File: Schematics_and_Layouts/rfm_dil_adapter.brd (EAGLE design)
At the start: 31.8 x 22.9 mm, 17 parts

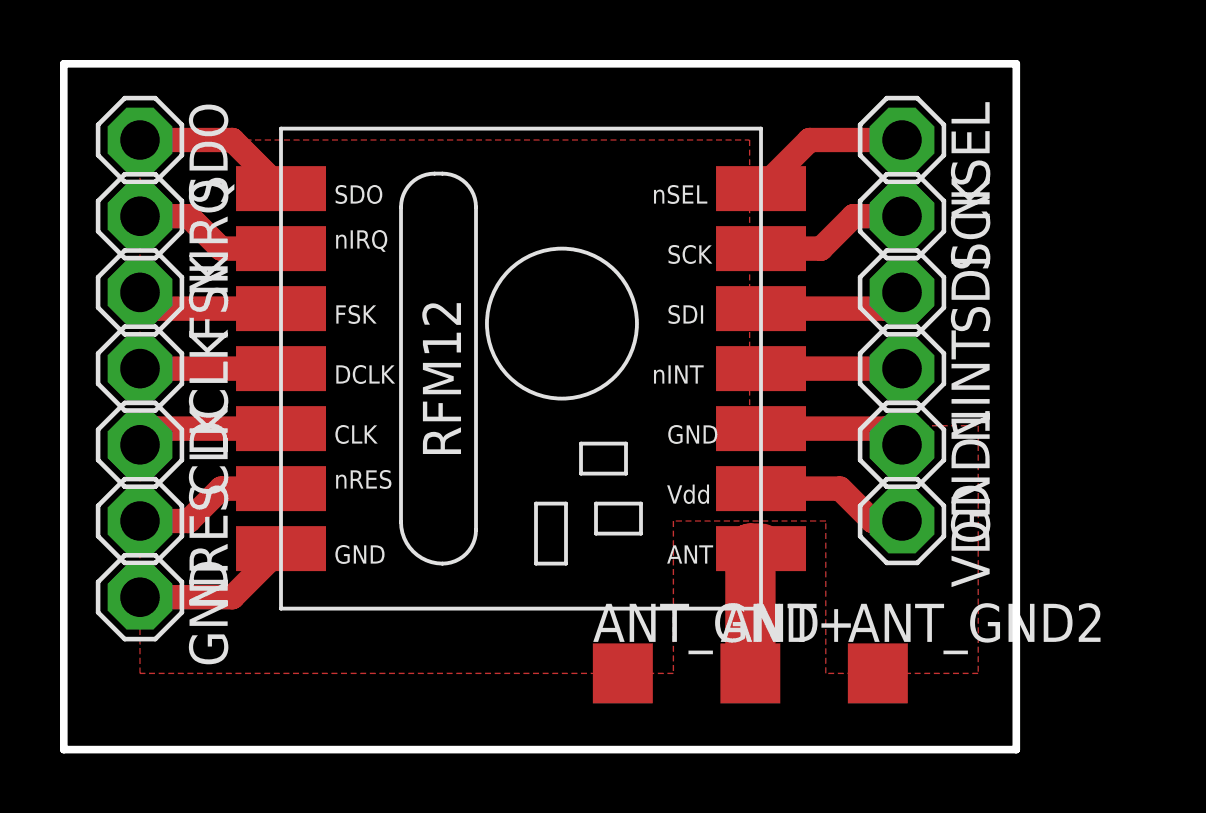
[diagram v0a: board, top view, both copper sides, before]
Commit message: Added Gerber Files
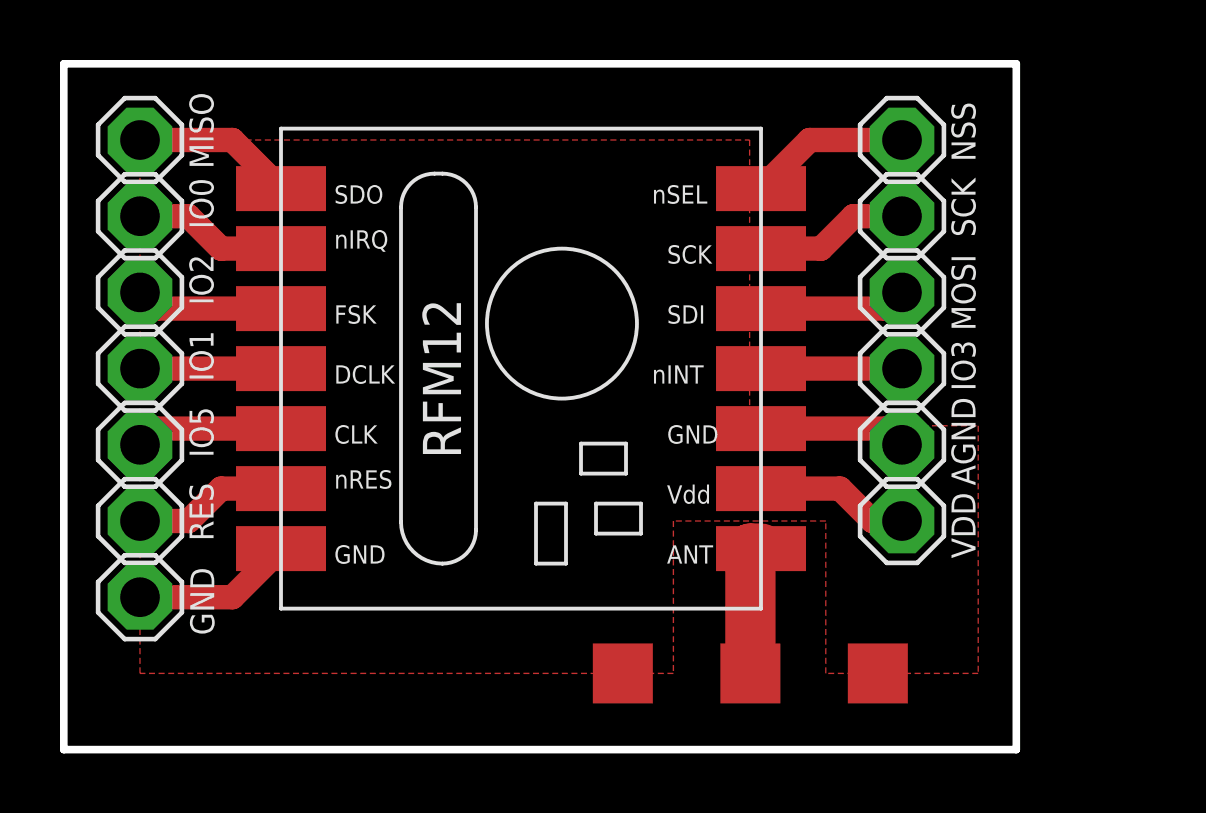
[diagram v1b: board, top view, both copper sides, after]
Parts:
- renumbered CLK to IO5, DCLK to IO1, FSK to IO2, GND1 to AGND, NINT to IO3, NIRQ to IO0, NRES to RES, NSEL to NSS, SDI to MOSI, SDO to MISO
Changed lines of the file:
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@@
 <?xml version="1.0" encoding="utf-8"?>
 <!DOCTYPE eagle SYSTEM "eagle.dtd">
-<eagle version="6.3">
+<eagle version="6.6.0">
 <drawing>
 <settings>
@@
 <setting verticaltext="up"/>
 </settings>
-<grid distance="1.27" unitdist="mm" unit="mm" style="lines" multiple="1" display="yes" altdistance="25" altunitdist="mil" altunit="mil"/>
+<grid distance="1.27" unitdist="mm" unit="mm" style="lines" multiple="1" display="yes" altdistance="12.5" altunitdist="mil" altunit="mil"/>
 <layers>
 <layer number="1" name="Top" color="4" fill="1" visible="yes" active="yes"/>
@@
 </autorouter>
 <elements>
-<element name="U$1" library="fp" package="RFM12_Z" value="RFM12_Z" x="15.24" y="12.7" rot="R270"/>
-<element name="CLK" library="solpad" package="SE13" value="SE13" x="2.54" y="10.16" rot="R270"/>
-<element name="DCLK" library="solpad" package="SE13" value="SE13" x="2.54" y="12.7" rot="R270"/>
-<element name="FSK" library="solpad" package="SE13" value="SE13" x="2.54" y="15.24" rot="R270"/>
-<element name="SDI" library="solpad" package="SE13" value="SE13" x="27.94" y="15.24" rot="R270"/>
-<element name="SDO" library="solpad" package="SE13" value="SE13" x="2.54" y="20.32" rot="R270"/>
-<element name="SCK" library="solpad" package="SE13" value="SE13" x="27.94" y="17.78" rot="R270"/>
-<element name="NSEL" library="solpad" package="SE13" value="SE13" x="27.94" y="20.32" rot="R270"/>
-<element name="GND" library="solpad" package="SE13" value="SE13" x="2.54" y="5.08" rot="R270"/>
-<element name="GND1" library="solpad" package="SE13" value="SE13" x="27.94" y="10.16" rot="R270"/>
-<element name="NRES" library="solpad" package="SE13" value="SE13" x="2.54" y="7.62" rot="R270"/>
-<element name="NIRQ" library="solpad" package="SE13" value="SE13" x="2.54" y="17.78" rot="R270"/>
-<element name="NINT" library="solpad" package="SE13" value="SE13" x="27.94" y="12.7" rot="R270"/>
-<element name="VDD" library="solpad" package="SE13" value="SE13" x="27.94" y="7.62" rot="R270"/>
-<element name="ANT+" library="testpad" package="TP20SQ" value="PTR1TP20SQ" x="22.885" y="2.54">
-<attribute name="TP_SIGNAL_NAME" value="" x="22.885" y="2.54" size="1.778" layer="27" display="off"/>
-</element>
-<element name="ANT_GND" library="testpad" package="TP20SQ" value="PTR1TP20SQ" x="18.635" y="2.54">
-<attribute name="TP_SIGNAL_NAME" value="" x="18.635" y="2.54" size="1.778" layer="27" display="off"/>
-</element>
-<element name="ANT_GND2" library="testpad" package="TP20SQ" value="PTR1TP20SQ" x="27.135" y="2.54">
-<attribute name="TP_SIGNAL_NAME" value="" x="27.135" y="2.54" size="1.778" layer="27" display="off"/>
+<element name="U$1" library="fp" package="RFM12_Z" value="RFM12_Z" x="15.24" y="12.7" smashed="yes" rot="R270"/>
+<element name="IO5" library="solpad" package="SE13" value="SE13" x="2.54" y="10.16" smashed="yes" rot="R270">
+<attribute name="NAME" x="4.191" y="11.43" size="0.8" layer="25" font="vector" ratio="20" rot="R270"/>
+</element>
+<element name="IO1" library="solpad" package="SE13" value="SE13" x="2.54" y="12.7" smashed="yes" rot="R270">
+<attribute name="NAME" x="4.191" y="13.97" size="0.8" layer="25" font="vector" ratio="20" rot="R270"/>
+</element>
+<element name="IO2" library="solpad" package="SE13" value="SE13" x="2.54" y="15.24" smashed="yes" rot="R270">
+<attribute name="NAME" x="4.191" y="16.51" size="0.8" layer="25" font="vector" ratio="20" rot="R270"/>
+</element>
+<element name="MOSI" library="solpad" package="SE13" value="SE13" x="27.94" y="15.24" smashed="yes" rot="R270">
+<attribute name="NAME" x="29.591" y="16.51" size="0.8" layer="25" font="vector" ratio="20" rot="R270"/>
+</element>
+<element name="MISO" library="solpad" package="SE13" value="SE13" x="2.54" y="20.32" smashed="yes" rot="R270">
+<attribute name="NAME" x="4.191" y="21.9075" size="0.8" layer="25" font="vector" ratio="20" rot="R270"/>
+</element>
+<element name="SCK" library="solpad" package="SE13" value="SE13" x="27.94" y="17.78" smashed="yes" rot="R270">
+<attribute name="NAME" x="29.591" y="19.05" size="0.8" layer="25" font="vector" ratio="20" rot="R270"/>
+</element>
+<element name="NSS" library="solpad" package="SE13" value="SE13" x="27.94" y="20.32" smashed="yes" rot="R270">
+<attribute name="NAME" x="29.591" y="21.59" size="0.8" layer="25" font="vector" ratio="20" rot="R270"/>
+</element>
+<element name="GND" library="solpad" package="SE13" value="SE13" x="2.54" y="5.08" smashed="yes" rot="R270">
+<attribute name="NAME" x="5.0165" y="3.81" size="0.8" layer="25" font="vector" ratio="20" rot="R90"/>
+</element>
+<element name="AGND" library="solpad" package="SE13" value="SE13" x="27.94" y="10.16" smashed="yes" rot="R270">
+<attribute name="NAME" x="29.591" y="11.7475" size="0.8" layer="25" font="vector" ratio="20" rot="R270"/>
+</element>
+<element name="RES" library="solpad" package="SE13" value="SE13" x="2.54" y="7.62" smashed="yes" rot="R270">
+<attribute name="NAME" x="4.191" y="8.89" size="0.8" layer="25" font="vector" ratio="20" rot="R270"/>
+</element>
+<element name="IO0" library="solpad" package="SE13" value="SE13" x="2.54" y="17.78" smashed="yes" rot="R270">
+<attribute name="NAME" x="4.191" y="19.05" size="0.8" layer="25" font="vector" ratio="20" rot="R270"/>
+</element>
+<element name="IO3" library="solpad" package="SE13" value="SE13" x="27.94" y="12.7" smashed="yes" rot="R270">
+<attribute name="NAME" x="29.591" y="13.6525" size="0.8" layer="25" font="vector" ratio="20" rot="R270"/>
+</element>
+<element name="VDD" library="solpad" package="SE13" value="SE13" x="27.94" y="7.62" smashed="yes" rot="R270">
+<attribute name="NAME" x="29.591" y="8.5725" size="0.8" layer="25" font="vector" ratio="20" rot="R270"/>
+</element>
+<element name="ANT+" library="testpad" package="TP20SQ" value="PTR1TP20SQ" x="22.885" y="2.54" smashed="yes">
+<attribute name="TP_SIGNAL_NAME" value="" x="22.885" y="0" size="1" layer="37"/>
+</element>
+<element name="ANT_GND" library="testpad" package="TP20SQ" value="PTR1TP20SQ" x="18.635" y="2.54" smashed="yes">
+<attribute name="TP_SIGNAL_NAME" value="" x="18.635" y="0" size="1" layer="37"/>
+</element>
+<element name="ANT_GND2" library="testpad" package="TP20SQ" value="PTR1TP20SQ" x="27.135" y="2.54" smashed="yes">
+<attribute name="TP_SIGNAL_NAME" value="" x="27.135" y="0" size="1" layer="37"/>
 </element>
 </elements>
@@
 <signal name="N$1">
 <contactref element="U$1" pad="CLK"/>
-<contactref element="CLK" pad="MP"/>
+<contactref element="IO5" pad="MP"/>
 <wire x1="2.54" y1="10.16" x2="3.08" y2="10.7" width="0.8128" layer="1"/>
 <wire x1="3.08" y1="10.7" x2="7.24" y2="10.7" width="0.8128" layer="1"/>
@@
 <signal name="N$2">
 <contactref element="U$1" pad="DCLK"/>
-<contactref element="DCLK" pad="MP"/>
+<contactref element="IO1" pad="MP"/>
 <wire x1="2.54" y1="12.7" x2="7.24" y2="12.7" width="0.8128" layer="1"/>
 </signal>
 <signal name="N$3">
 <contactref element="U$1" pad="FSK"/>
-<contactref element="FSK" pad="MP"/>
+<contactref element="IO2" pad="MP"/>
 <wire x1="2.54" y1="15.24" x2="3.08" y2="14.7" width="0.8128" layer="1"/>
 <wire x1="3.08" y1="14.7" x2="7.24" y2="14.7" width="0.8128" layer="1"/>
@@
 <signal name="N$4">
 <contactref element="U$1" pad="SDI"/>
-<contactref element="SDI" pad="MP"/>
+<contactref element="MOSI" pad="MP"/>
 <wire x1="27.94" y1="15.24" x2="27.4" y2="14.7" width="0.8128" layer="1"/>
 <wire x1="27.4" y1="14.7" x2="23.240003125" y2="14.7" width="0.8128" layer="1"/>
@@
 <signal name="N$5">
 <contactref element="U$1" pad="SDO"/>
-<contactref element="SDO" pad="MP"/>
+<contactref element="MISO" pad="MP"/>
 <wire x1="2.54" y1="20.32" x2="5.62" y2="20.32" width="0.8128" layer="1"/>
 <wire x1="5.62" y1="20.32" x2="7.239996875" y2="18.700003125" width="0.8128" layer="1"/>
@@
 <signal name="N$7">
 <contactref element="U$1" pad="NSEL"/>
-<contactref element="NSEL" pad="MP"/>
+<contactref element="NSS" pad="MP"/>
 <wire x1="27.94" y1="20.32" x2="24.86" y2="20.32" width="0.8128" layer="1"/>
 <wire x1="24.86" y1="20.32" x2="23.24" y2="18.7" width="0.8128" layer="1"/>
@@
 <signal name="N$11">
 <contactref element="U$1" pad="NRES"/>
-<contactref element="NRES" pad="MP"/>
+<contactref element="RES" pad="MP"/>
 <wire x1="2.54" y1="7.62" x2="4.159996875" y2="7.62" width="0.8128" layer="1"/>
 <wire x1="4.159996875" y1="7.62" x2="5.23999375" y2="8.699996875" width="0.8128" layer="1"/>
@@
 <signal name="N$12">
 <contactref element="U$1" pad="NIRQ"/>
-<contactref element="NIRQ" pad="MP"/>
+<contactref element="IO0" pad="MP"/>
 <wire x1="2.54" y1="17.78" x2="4.159996875" y2="17.78" width="0.8128" layer="1"/>
 <wire x1="4.159996875" y1="17.78" x2="5.23999375" y2="16.700003125" width="0.8128" layer="1"/>
@@
 <signal name="N$13">
 <contactref element="U$1" pad="NINT"/>
-<contactref element="NINT" pad="MP"/>
+<contactref element="IO3" pad="MP"/>
 <wire x1="27.94" y1="12.7" x2="23.24" y2="12.7" width="0.8128" layer="1"/>
 </signal>
@@
 <wire x1="5.62" y1="5.08" x2="7.24" y2="6.7" width="0.8128" layer="1"/>
 <contactref element="U$1" pad="GND1"/>
-<contactref element="GND1" pad="MP"/>
+<contactref element="AGND" pad="MP"/>
 <wire x1="27.94" y1="10.16" x2="27.4" y2="10.7" width="0.8128" layer="1"/>
 <wire x1="27.4" y1="10.7" x2="23.24" y2="10.7" width="0.8128" layer="1"/>
